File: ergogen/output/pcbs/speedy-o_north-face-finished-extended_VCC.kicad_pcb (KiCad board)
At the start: 2 copper layers, 148.6 x 108.6 mm, 96 parts

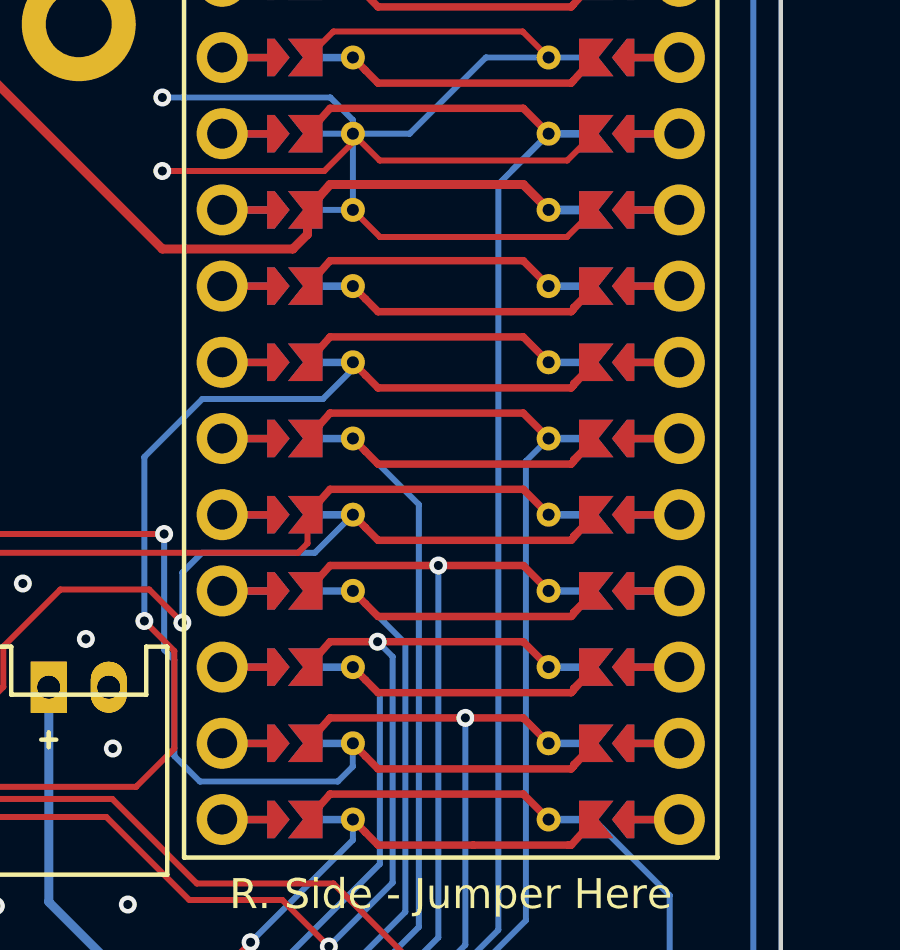
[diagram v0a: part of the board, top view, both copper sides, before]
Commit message: update pcb
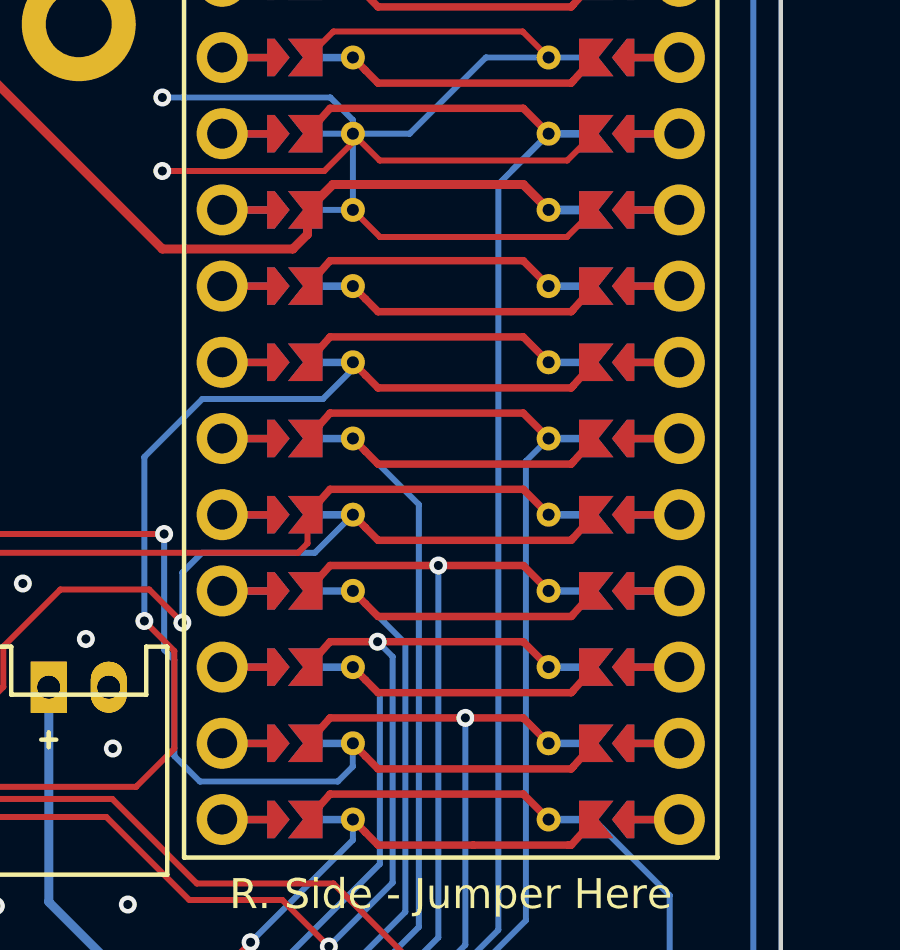
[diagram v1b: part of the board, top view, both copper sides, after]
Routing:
- net P8: track 177.5 -> 176.4 mm
- net P4: track 235.5 -> 234.5 mm
- net P2: track 12.0 -> 10.9 mm
- net P7: track 174.7 -> 173.7 mm
- net P6: track 182.2 -> 181.2 mm
- net P5: track 190.8 -> 189.8 mm
- net P3: track 235.4 -> 234.3 mm
- net VCC: track 736.2 -> 736.8 mm
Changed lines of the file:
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@@
 	)
 	(segment
+		(start 209.4844 85.35)
+		(end 208.6381 86.1963)
+		(width 0.3)
+		(layer "F.Cu")
+		(net 1)
+	)
+	(segment
 		(start 184.353 93.0063)
 		(end 182.6313 93.0063)
@@
 	)
 	(segment
-		(start 209.015 85.775)
-		(end 209.39 85.35)
-		(width 0.3)
-		(layer "F.Cu")
-		(net 1)
-	)
-	(segment
 		(start 155.1134 104.606)
 		(end 155.1131 104.6063)
@@
 	)
 	(segment
-		(start 210.7553 85.35)
-		(end 215.83 85.35)
-		(width 0.3)
-		(layer "F.Cu")
-		(net 1)
-	)
-	(segment
 		(start 118.117648 105)
 		(end 115.015103 108.102545)
@@
 	)
 	(segment
+		(start 209.4844 85.35)
+		(end 215.83 85.35)
+		(width 0.3)
+		(layer "F.Cu")
+		(net 1)
+	)
+	(segment
 		(start 181.05 141.7)
 		(end 180.6632 142.0868)
@@
 	)
 	(segment
-		(start 209.39 85.35)
-		(end 210.7553 85.35)
-		(width 0.3)
-		(layer "F.Cu")
-		(net 1)
-	)
-	(segment
 		(start 149.7131 89.0063)
 		(end 149.7131 90.2056)
@@
 	)
 	(segment
-		(start 218.1881 98.8963)
-		(end 217.4922 99.5922)
-		(width 0.2)
-		(layer "F.Cu")
-		(net 31)
-	)
-	(segment
 		(start 175.2937 127.4063)
 		(end 180.4131 127.4063)
@@
 	)
 	(segment
-		(start 217.4922 99.5922)
-		(end 217.4922 99.6804)
-		(width 0.2)
-		(layer "F.Cu")
-		(net 31)
-	)
-	(segment
 		(start 106.251583 130.8)
 		(end 107.258358 129.793225)
@@
 	)
 	(segment
-		(start 218.1881 101.4363)
-		(end 217.4922 102.1322)
-		(width 0.2)
-		(layer "F.Cu")
-		(net 33)
-	)
-	(segment
 		(start 218.19 101.44)
 		(end 217.4922 102.2204)
@@
 	)
 	(segment
-		(start 217.4922 102.1322)
-		(end 217.4922 102.2204)
-		(width 0.2)
-		(layer "F.Cu")
-		(net 33)
-	)
-	(segment
 		(start 163.3148 108.4063)
 		(end 166.6 111.6915)
@@
 	)
 	(segment
-		(start 218.1881 103.9763)
-		(end 217.4922 104.6722)
-		(width 0.2)
-		(layer "F.Cu")
-		(net 35)
-	)
-	(segment
 		(start 162.4068 91.4)
 		(end 162.4131 91.4063)
@@
 	)
 	(segment
-		(start 217.4922 104.6722)
-		(end 217.4922 104.7604)
-		(width 0.2)
-		(layer "F.Cu")
-		(net 35)
-	)
-	(segment
 		(start 169.4 97.4)
 		(end 171.6 97.4)
@@
 	)
 	(segment
-		(start 218.1881 91.2763)
-		(end 217.4922 91.9722)
-		(width 0.2)
-		(layer "F.Cu")
-		(net 62)
-	)
-	(segment
 		(start 94.574265 124.4)
 		(end 92.853052 122.678787)
@@
 	)
 	(segment
-		(start 217.4922 91.9722)
-		(end 217.4922 92.0604)
-		(width 0.2)
-		(layer "F.Cu")
-		(net 62)
-	)
-	(segment
 		(start 99.6 153.2)
 		(end 97.584952 155.215048)
@@
 	)
 	(segment
-		(start 217.4922 94.5122)
-		(end 217.4922 94.6004)
-		(width 0.2)
-		(layer "F.Cu")
-		(net 63)
-	)
-	(segment
 		(start 123.2 138.6041)
 		(end 124.6959 138.6041)
@@
 	)
 	(segment
-		(start 218.1881 93.8163)
-		(end 217.4922 94.5122)
-		(width 0.2)
-		(layer "F.Cu")
-		(net 63)
-	)
-	(segment
 		(start 117 151.2)
 		(end 117.2 151)
@@
 	)
 	(segment
-		(start 217.4922 97.0522)
-		(end 217.4922 97.1404)
-		(width 0.2)
-		(layer "F.Cu")
-		(net 64)
-	)
-	(segment
 		(start 194.45 103.6)
 		(end 195.45 102.6)
@@
 	)
 	(segment
-		(start 218.1881 96.3563)
-		(end 217.4922 97.0522)
-		(width 0.2)
-		(layer "F.Cu")
-		(net 64)
-	)
-	(segment
 		(start 131.1381 134.9563)
 		(end 133.8286 137.6468)
@@
 	)
 	(segment
-		(start 218.1881 88.7363)
-		(end 217.4922 89.4322)
-		(width 0.2)
-		(layer "F.Cu")
-		(net 70)
-	)
-	(segment
 		(start 217.43 89.59)
 		(end 210.99 89.59)
@@
 		(layer "F.Cu")
 		(net 70)
-	)
-	(segment
-		(start 217.4922 89.4322)
-		(end 217.4922 89.5204)
-		(width 0.2)
-		(layer "F.Cu")
-		(net 70)
